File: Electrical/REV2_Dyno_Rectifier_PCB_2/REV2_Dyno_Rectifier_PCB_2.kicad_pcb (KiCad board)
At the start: 2 copper layers, 25 x 22 mm, 35 parts, among them J1 Dynamo Input, J2 Barrel_Jack_MountingPin, U1 TPS63070RNMR, U2 PAM2803AAF095

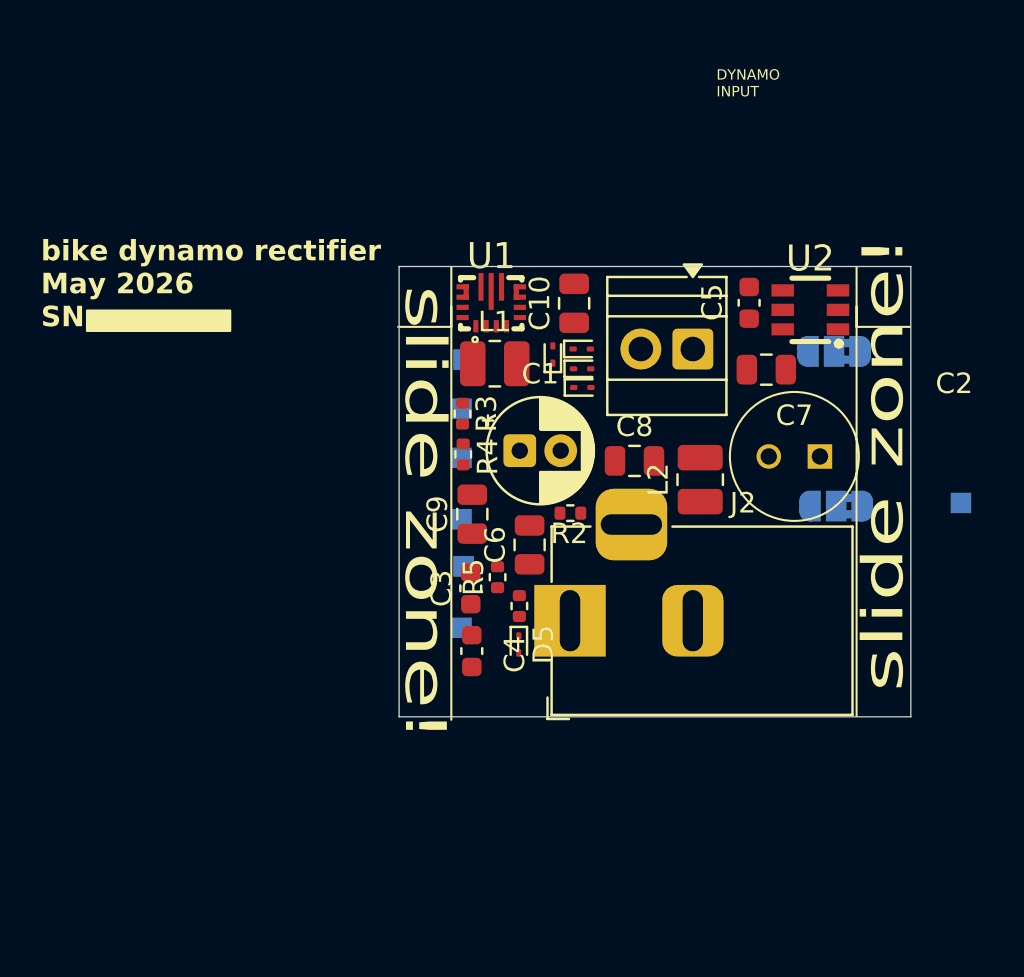
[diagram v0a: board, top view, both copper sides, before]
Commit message: sent off rectifier PCB and the Light PCB off to JLCPCB tonight
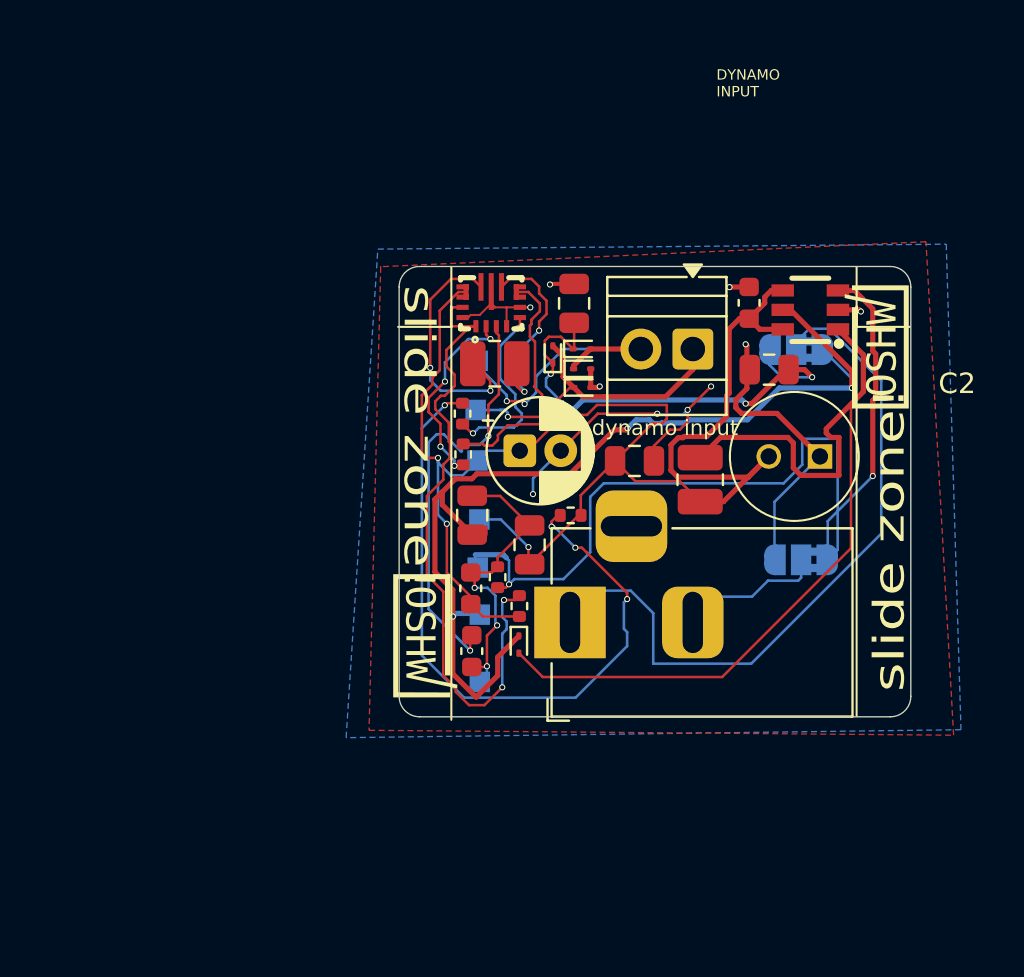
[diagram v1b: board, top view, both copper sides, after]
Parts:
- added REF**: oshw mark, william_custom:oshw mark, F.Cu at (79.5, 37.6)
- added REF**: oshw mark, william_custom:oshw mark, F.Cu at (53.6, 52.9)
- added REF**: oshw mark, william_custom:oshw mark, B.Cu at (73.4, 54.0)
- R5: value 2.7 -> 1.8
- moved TP6 24.1 mm to (58.2, 51.3)
- moved JP2 3.13 mm to (73.9, 48.6)
- moved TP7 2.80 mm to (58.2, 54.5)
- moved JP1 1.85 mm to (73.7, 38.3)
- moved TP4 0.87 mm to (58.2, 46.6)
- moved TP3 0.79 mm to (58.1, 43.7)
- moved TP1 0.69 mm to (58.1, 38.9)
- moved TP5 0.69 mm to (58.1, 49.0)
- moved TP2 0.69 mm to (58.0, 41.3)
- moved C2 0.14 mm to (72.3, 39.3)
- moved R2 0.11 mm to (62.6, 46.4)
- moved J2 0.08 mm to (62.6, 51.6)
- moved C9 0.05 mm to (57.8, 46.4)
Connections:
- J2 pad 1: Out_Sleeve -> Out_Tip
- J2 pad 2: Out_Tip -> Out_Sleeve
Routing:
- net 2.7V: track 0.00 -> 62.5 mm, vias 0 -> 3
- net GND: track 0.00 -> 54.8 mm, vias 0 -> 13
- net Rectified: track 0.00 -> 52.7 mm, vias 0 -> 6
- net V_out: track 0.00 -> 49.5 mm, vias 0 -> 3
- net FB: track 0.00 -> 47.1 mm, vias 0 -> 2
- net Net-(D5-A): track 0.00 -> 43.9 mm
- net Out_Tip: track 0.00 -> 34.7 mm
- net Net-(R2-Pad2): track 0.00 -> 34.1 mm, vias 0 -> 4
- net Net-(U1-EN): track 0.00 -> 31.5 mm, vias 0 -> 2
- net Net-(U1-Vaux): track 0.00 -> 21.3 mm, vias 0 -> 2
- net Raw_Input_-: track 0.00 -> 15.9 mm, vias 0 -> 1
- net Raw_Input_+: track 0.00 -> 14.5 mm, vias 0 -> 2
- net Net-(U1-L1): track 0.00 -> 12.1 mm, vias 0 -> 2
- net Net-(U1-L2): track 0.00 -> 9.98 mm, vias 0 -> 2
- net Net-(U1-PG): track 0.00 -> 9.77 mm, vias 0 -> 4
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- added copper zone on B.Cu, net GND
- added copper zone on F.Cu, net GND
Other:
- outline, holes or cut-outs redrawn
- board text added: "2.7V"
- board text added: "FB"
- board text added: "GND"
- board text added: "Rev. 2 - May 2026"
- board text added: "US002271"
- board text added: "contactless bike dynamo rectifier"
- board text added: "dynamo input"
- board text added: "freakylamps w. kennedy SN:"
- board text added: "out"
- board text added: "raw in +"
- board text added: "raw in -"
- board text added: "rectified"
- board text added: "regulated"
- board text removed: "bike dynamo rectifier May 2026 SN:"
